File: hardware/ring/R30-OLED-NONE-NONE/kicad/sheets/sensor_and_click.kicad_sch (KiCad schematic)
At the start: 7 parts, among them SW1 5mm 200gf dome, U2 PAW3204DB-TJ3L

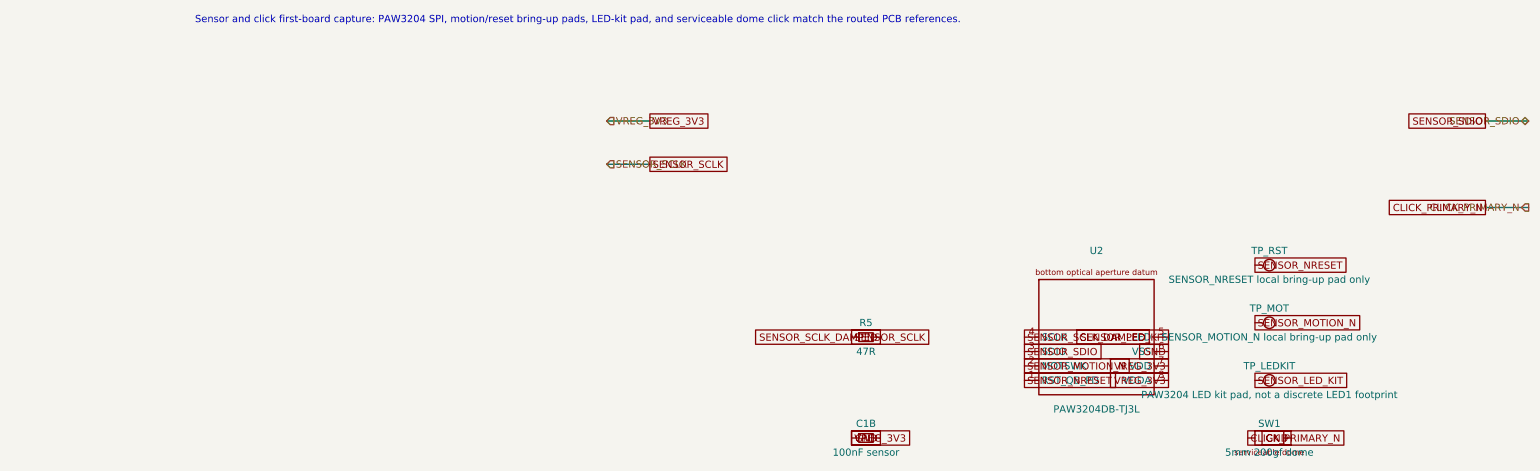
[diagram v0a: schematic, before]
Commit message: feat(r30): close optical ring fabrication review gate
Sensing mechanism: PAW3204 optical sensor with matched lens/emitter path. Form factor and angle: R30-OLED-NONE-NONE fingertip ring, 30 deg optical posture. Intended use case: offline BLE HID pointing/accessibility ring. BOM estimate: remains under the sub- prototype target in the active R30 BOM.
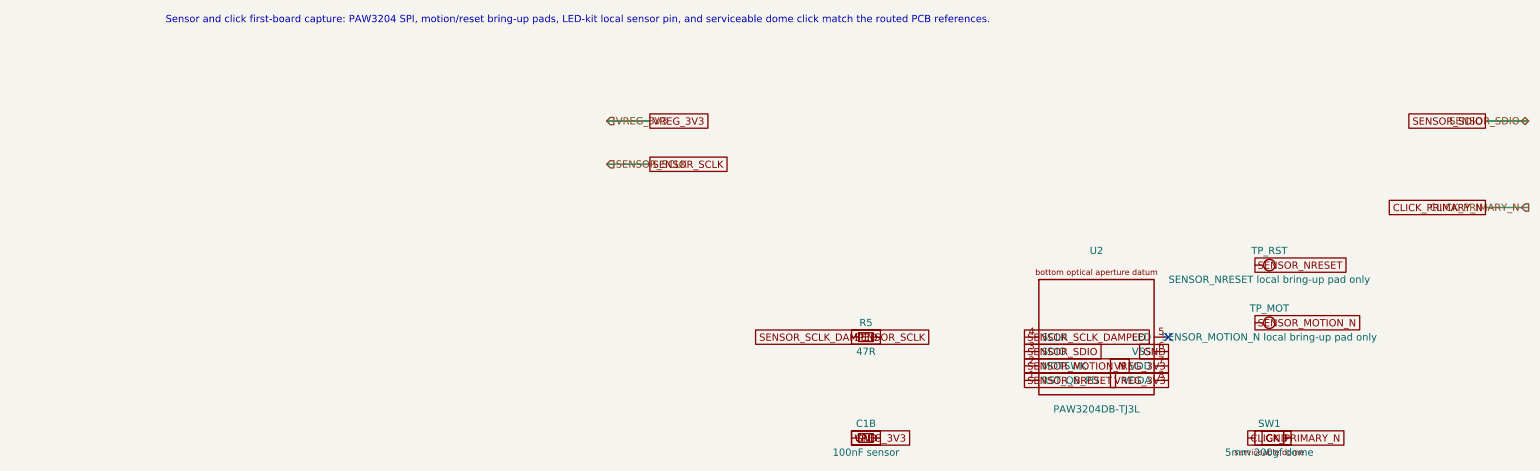
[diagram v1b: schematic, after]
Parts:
- removed TP_LEDKIT: PAW3204 LED kit pad, not a discrete LED1 footprint, TestPoint:TestPoint_Pad_D1.0mm, symbol PowerFinger:TESTPAD_1MM
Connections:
- net SENSOR_LED_KIT: no longer names the net of U2.5 (LED)
- no-connect marks 0 -> 1
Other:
- note added: "Sensor and click first-board capture: PAW3204 SPI, motion/reset bring-up pads, LED-kit local sensor pin, and serviceable dome click match the routed PCB references."
- note removed: "Sensor and click first-board capture: PAW3204 SPI, motion/reset bring-up pads, LED-kit pad, and serviceable dome click match the routed PCB references."
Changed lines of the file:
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@@
   (generator_version "0.1")
   (paper "A4")
-  (text "Sensor and click first-board capture: PAW3204 SPI, motion/reset bring-up pads, LED-kit pad, and serviceable dome click match the routed PCB references."
+  (text "Sensor and click first-board capture: PAW3204 SPI, motion/reset bring-up pads, LED-kit local sensor pin, and serviceable dome click match the routed PCB references."
     (at 20.32 20.32 0)
     (effects (font (size 1.27 1.27)))
@@
     )
   )
-  (symbol (lib_id "PowerFinger:TESTPAD_1MM") (at 142.24 83.82 0) (unit 1)
-    (in_bom yes) (on_board yes) (dnp no)
-    (property "Reference" "TP_LEDKIT" (at 142.24 81.28 0)
-      (effects (font (size 1.27 1.27)))
-    )
-    (property "Value" "PAW3204 LED kit pad, not a discrete LED1 footprint" (at 142.24 86.36 0)
-      (effects (font (size 1.27 1.27)))
-    )
-    (property "Footprint" "TestPoint:TestPoint_Pad_D1.0mm" (at 142.24 88.9 0)
-      (effects (font (size 1.27 1.27)) hide)
-    )
-    (pin "1")
-    (instances
-      (project "r30_oled_none_none"
-        (path "/" (reference "TP_LEDKIT") (unit 1))
-      )
-    )
-  )
   (global_label "SENSOR_NRESET" (shape passive) (at 99.06 83.82 0) (effects (font (size 1.27 1.27))))
   (global_label "SENSOR_MOTION_N" (shape passive) (at 99.06 81.28 0) (effects (font (size 1.27 1.27))))
   (global_label "SENSOR_SDIO" (shape passive) (at 99.06 78.74 0) (effects (font (size 1.27 1.27))))
   (global_label "SENSOR_SCLK_DAMPED" (shape passive) (at 99.06 76.2 0) (effects (font (size 1.27 1.27))))
-  (global_label "SENSOR_LED_KIT" (shape passive) (at 124.46 76.2 180) (effects (font (size 1.27 1.27))))
+  (no_connect (at 124.46 76.2))
   (global_label "GND" (shape passive) (at 124.46 78.74 180) (effects (font (size 1.27 1.27))))
   (global_label "VREG_3V3" (shape passive) (at 124.46 81.28 180) (effects (font (size 1.27 1.27))))
@@
   (global_label "SENSOR_NRESET" (shape passive) (at 139.7 63.5 0) (effects (font (size 1.27 1.27))))
   (global_label "SENSOR_MOTION_N" (shape passive) (at 139.7 73.66 0) (effects (font (size 1.27 1.27))))
-  (global_label "SENSOR_LED_KIT" (shape passive) (at 139.7 83.82 0) (effects (font (size 1.27 1.27))))
   (sheet_instances
     (path "/" (page "1"))
